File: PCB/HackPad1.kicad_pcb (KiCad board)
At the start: 2 copper layers, 68.5 x 88.5 mm, 26 parts, among them J1 Conn_01x04_Pin, SW1 SW_Push, SW10 RotaryEncoder, SW2 SW_Push, SW3 SW_Push, SW4 SW_Push, SW5 SW_Push, SW6 SW_Push, SW7 SW_Push, SW8 SW_Push, SW9 SW_Push, U1 MOUDLE-SEEEDUINO-XIAO

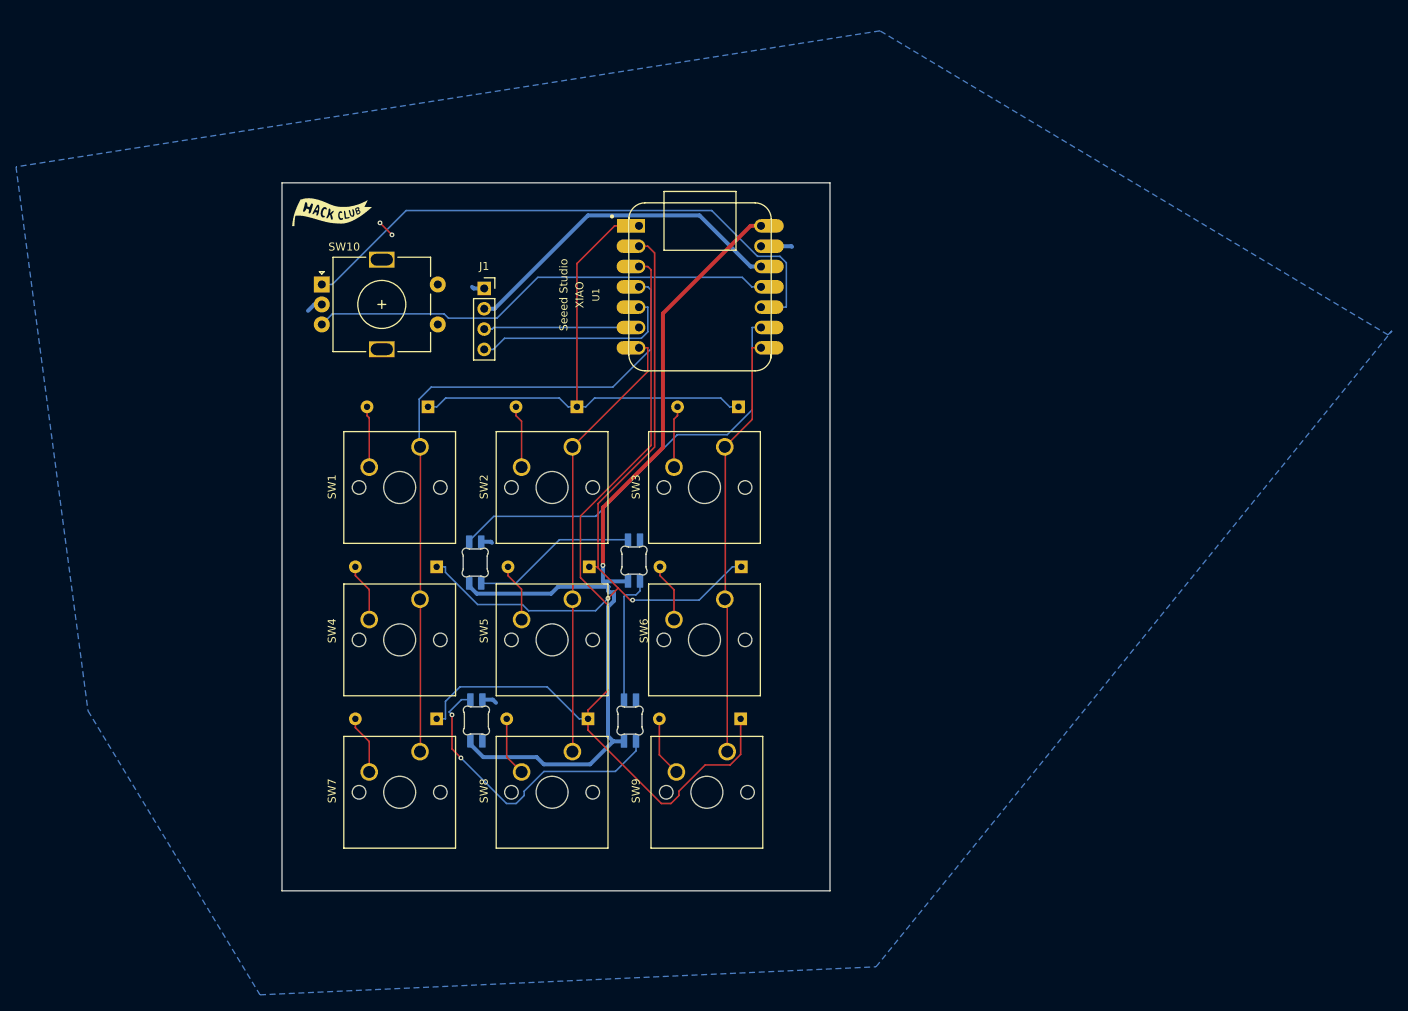
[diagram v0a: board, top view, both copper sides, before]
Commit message: Pcb routing
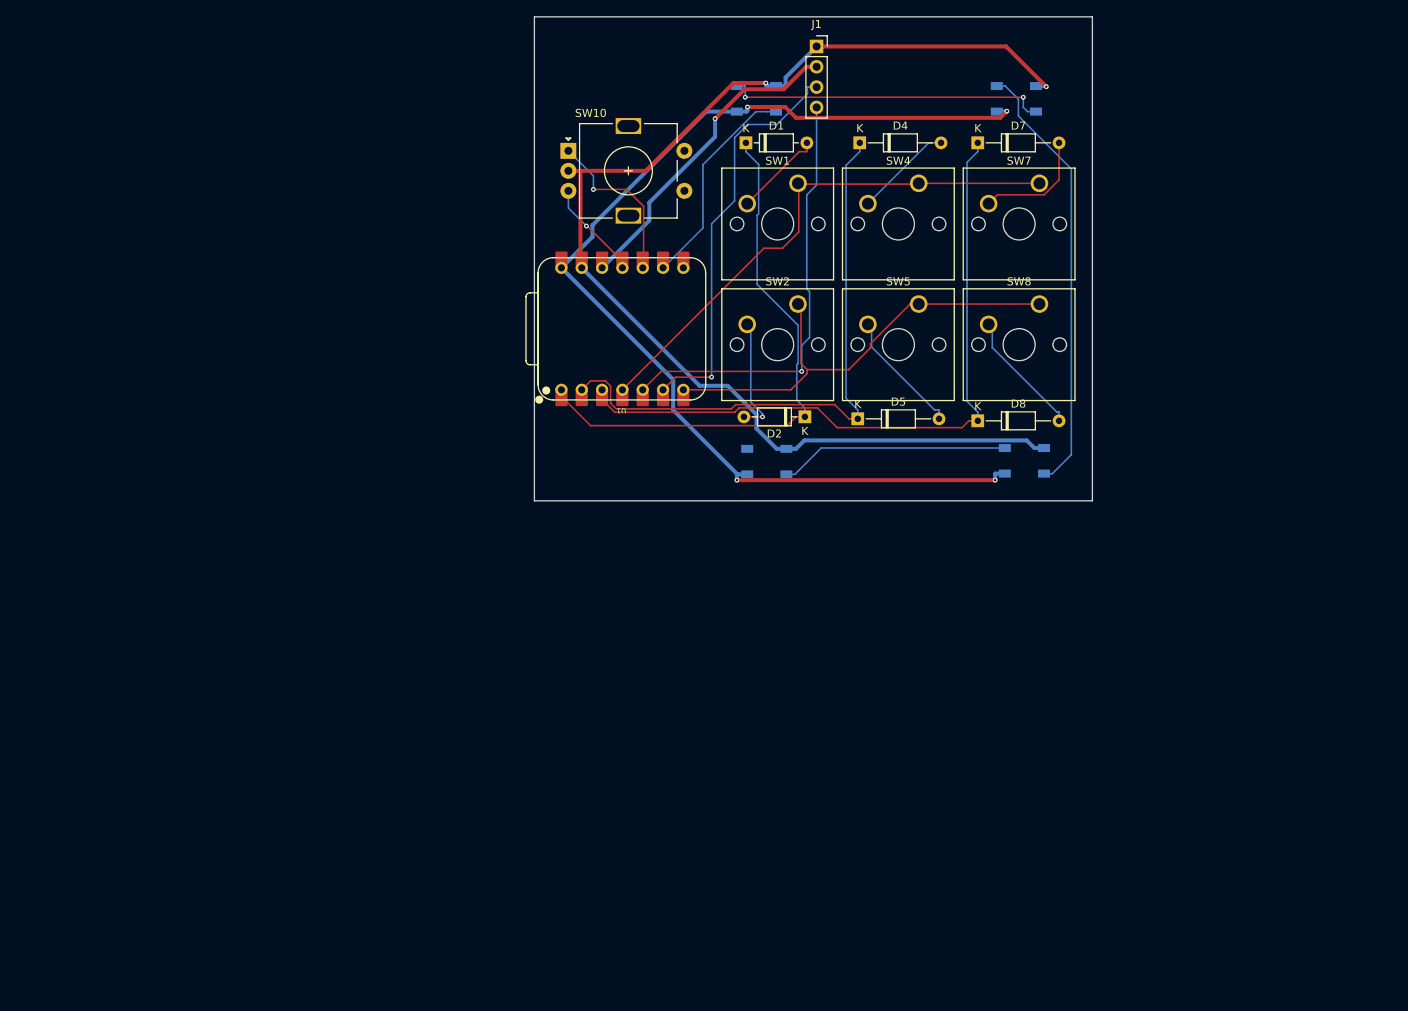
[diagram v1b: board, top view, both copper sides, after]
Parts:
- removed ?: , clipboard:f94af434-1fa3-4cc6-adfb-df3f992dc55a
- removed D3: D, Diode_THT:D_DO-35_SOD27_P7.62mm_Horizontal
- removed D6, D9: D, Diode_THT:D_DO-35_SOD27_P10.16mm_Horizontal
- removed SW3, SW6, SW9: SW_Push, Button_Switch_Keyboard:SW_Cherry_MX_1.00u_PCB
- D1, D2, D4, D5, D7, D8: moved to F.Cu
- D10, D11, D12, D13: footprint Keyboard_Parts:MX_SK6812MINI-E -> LED_SMD:LED_SK6812_PLCC4_5.0x5.0mm_P3.2mm; moved to B.Cu
- U1: footprint footprints:XIAO-Generic-Hybrid-14P-2.54-21X17.8MM -> New_XIAO_Series_Footprints:XIAO-SAMD21-DIP
- moved SW7 105.1 mm to (177.4, 67.1)
- moved D7 98.8 mm to (169.7, 62.0), turned to 0 degrees
- moved SW4 81.2 mm to (162.3, 67.1)
- moved SW8 80.9 mm to (177.4, 82.2)
- moved D11 78.3 mm to (174.6, 56.5), turned to 180 degrees
- moved D4 74.9 mm to (155.0, 62.0), turned to 0 degrees
- moved D10 70.6 mm to (142.1, 56.5), turned to 180 degrees
- moved D12 63.3 mm to (175.6, 101.8), turned to 180 degrees
- moved D8 61.3 mm to (169.7, 96.8), turned to 0 degrees
- moved SW1 57.6 mm to (147.2, 67.1)
- moved SW5 56.9 mm to (162.3, 82.2)
- moved D13 52.5 mm to (143.3, 101.8), turned to 180 degrees
- moved D1 51.7 mm to (140.7, 62.0), turned to 0 degrees
- moved J1 51.4 mm to (149.6, 50.0)
- moved D5 38.3 mm to (154.7, 96.5), turned to 0 degrees
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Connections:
- U1 pad 8: ROW3 -> unconnected-(U1-PB09_A7_D7_RX-Pad8)_0
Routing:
- net GND: track 13.0 -> 151.9 mm
- net ROW3: track 53.2 -> 0.00 mm
- net ENCA: track 73.3 -> 21.0 mm, vias 0 -> 1
- net ENCB: track 58.3 -> 12.5 mm, vias 0 -> 1
- net Net-(D11-DOUT): track 16.4 -> 55.0 mm
- net COL3: track 119.0 -> 86.3 mm
- net SCL: track 19.4 -> 52.1 mm, vias 0 -> 1
- net SDA: track 25.5 -> 55.7 mm, vias 0 -> 1
- net LED_DATA: track 53.7 -> 27.7 mm
- net +5V: track 118.3 -> 139.3 mm, vias 1 -> 4
- net Net-(D10-DOUT): track 20.6 -> 40.3 mm, vias 0 -> 2
- net COL2: track 93.5 -> 75.3 mm, vias 2 -> 0
- net ROW1: track 84.8 -> 67.3 mm
- net Net-(D12-DOUT): track 38.5 -> 28.7 mm, vias 2 -> 0
- net Net-(D5-A): track 7.29 -> 15.8 mm
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- removed copper zone on B.Cu, net GND
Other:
- board size 68.5 x 88.5 mm -> 69.8 x 60.5 mm

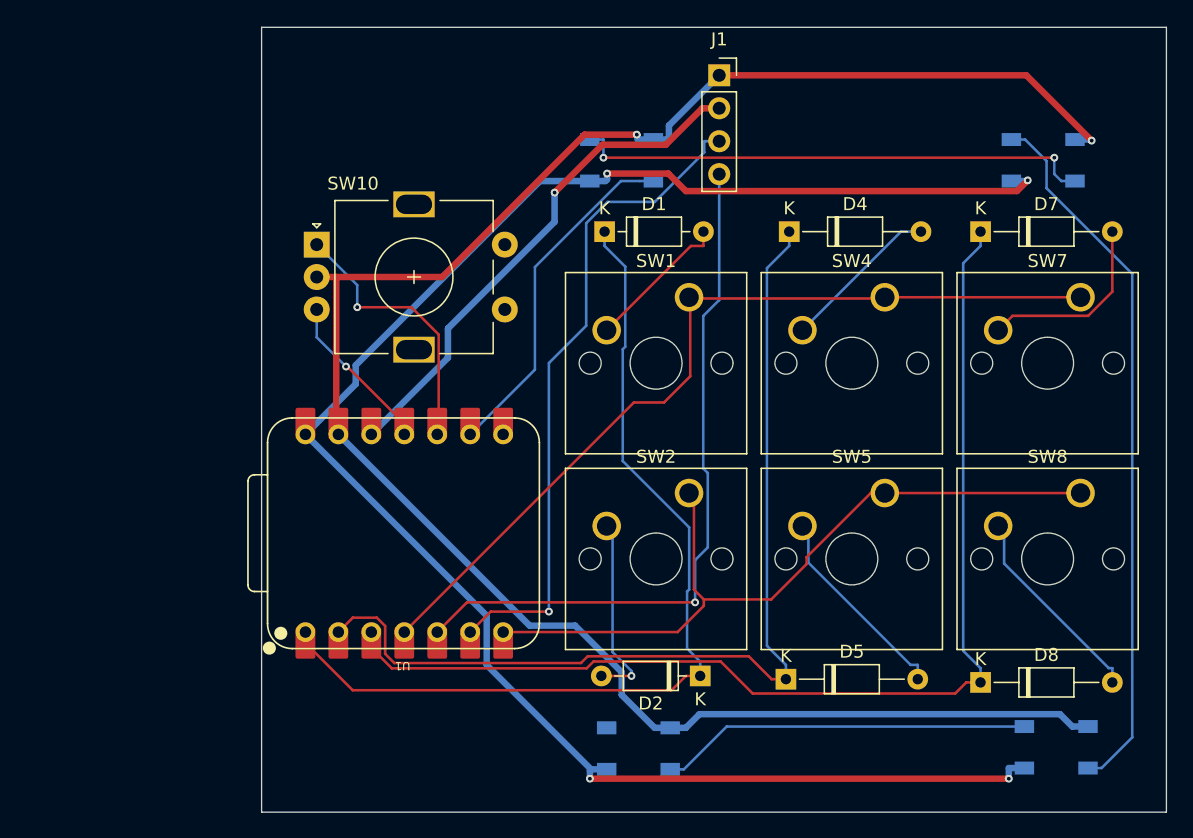
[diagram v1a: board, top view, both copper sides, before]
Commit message: Initial commit
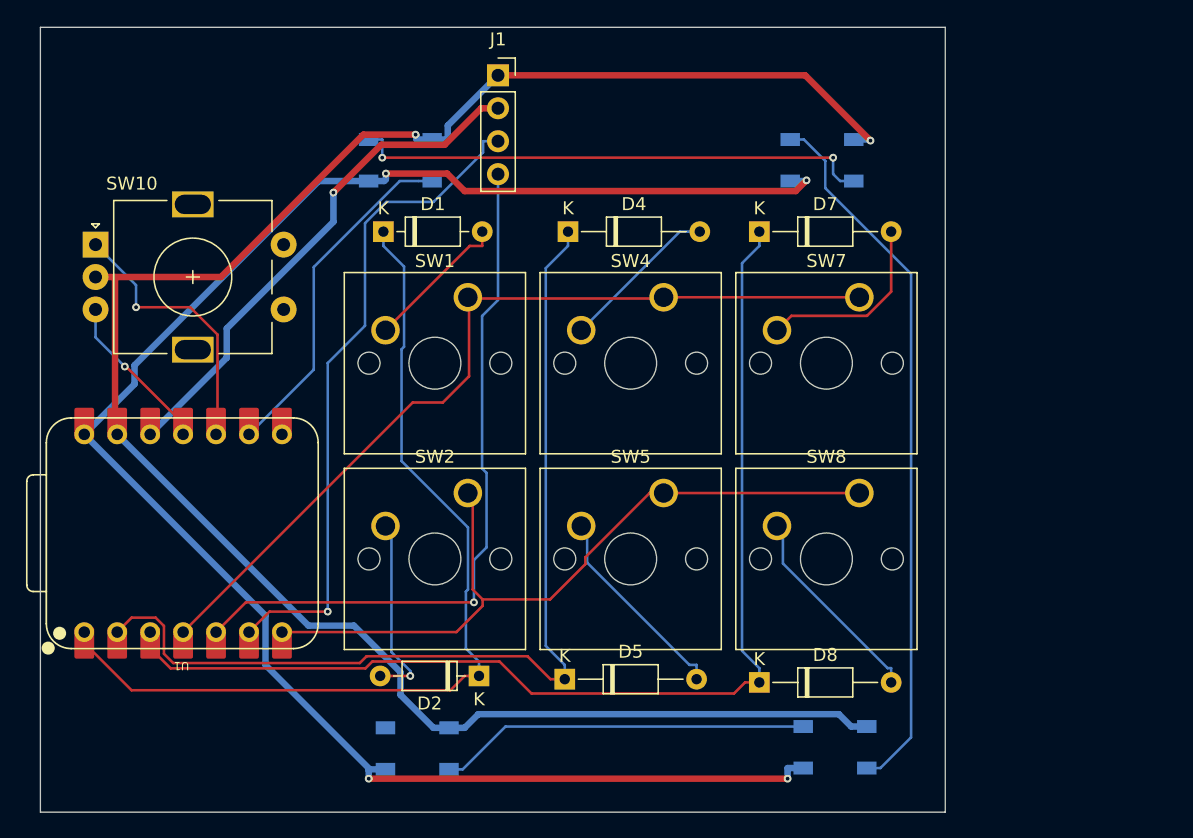
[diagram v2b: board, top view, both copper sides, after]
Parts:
- moved D1 17.1 mm to (123.7, 62.0)
- moved D10 17.1 mm to (125.0, 56.5)
- moved D11 17.1 mm to (157.5, 56.5)
- moved D12 17.1 mm to (158.5, 101.8)
- moved D2 17.1 mm to (131.1, 96.2)
- moved D4 17.1 mm to (137.9, 62.0)
- moved D5 17.1 mm to (137.7, 96.5)
- moved D7 17.1 mm to (152.7, 62.0)
- moved D8 17.1 mm to (152.7, 96.8)
- moved SW1 17.1 mm to (130.2, 67.1)
- moved SW2 17.1 mm to (130.2, 82.2)
- moved SW4 17.1 mm to (145.3, 67.1)
- moved SW5 17.1 mm to (145.3, 82.2)
- moved SW7 17.1 mm to (160.4, 67.1)
- moved SW8 17.1 mm to (160.4, 82.2)
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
